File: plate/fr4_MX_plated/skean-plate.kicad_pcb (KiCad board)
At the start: 2 copper layers, 153.2 x 95.3 mm, 32 parts, among them K1 KEYSW, K10 KEYSW, K11 KEYSW, K12 KEYSW, K13 KEYSW, K14 KEYSW, K15 KEYSW, K16 KEYSW, K17 KEYSW, K18 KEYSW, K19 KEYSW, K2 KEYSW, K20 KEYSW, K21 KEYSW, K22 KEYSW, K3 KEYSW, K4 KEYSW, K5 KEYSW, K6 KEYSW, K7 KEYSW, K8 KEYSW, K9 KEYSW

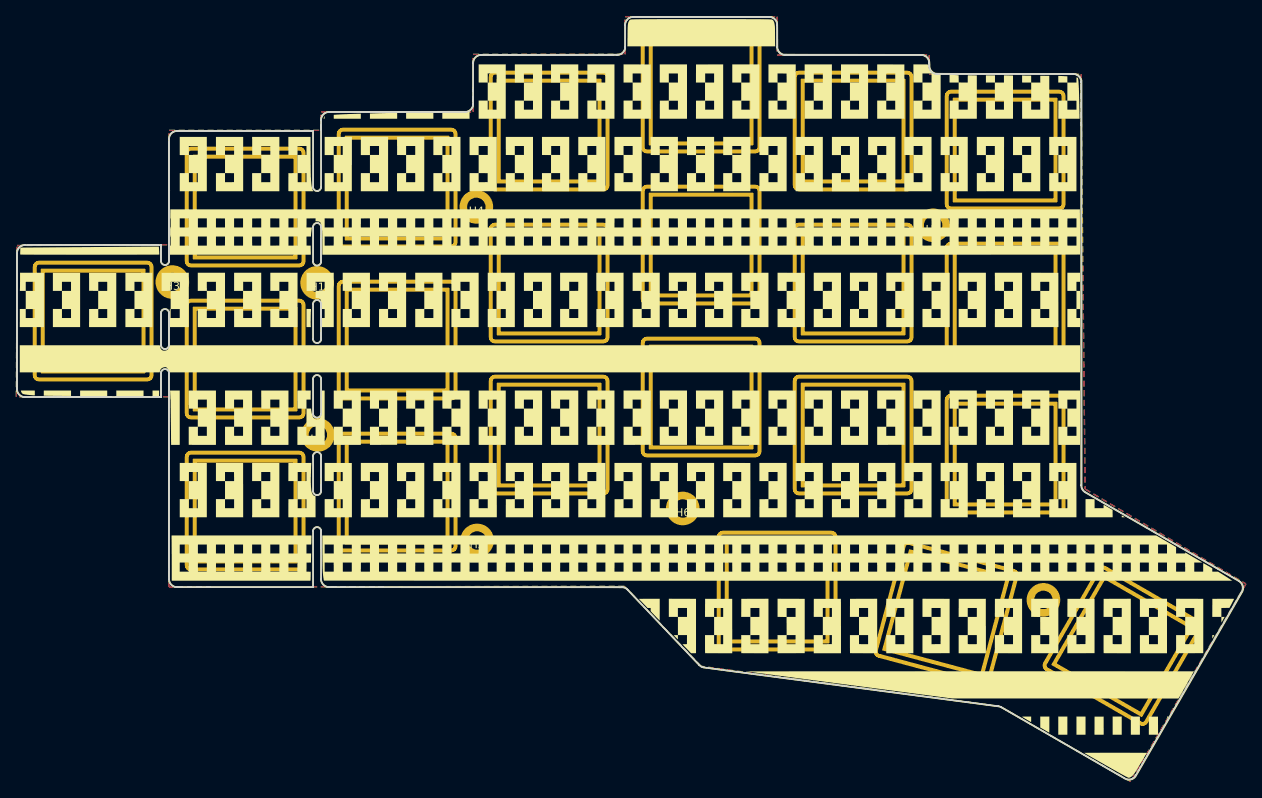
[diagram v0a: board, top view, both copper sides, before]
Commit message: V0.3 case files
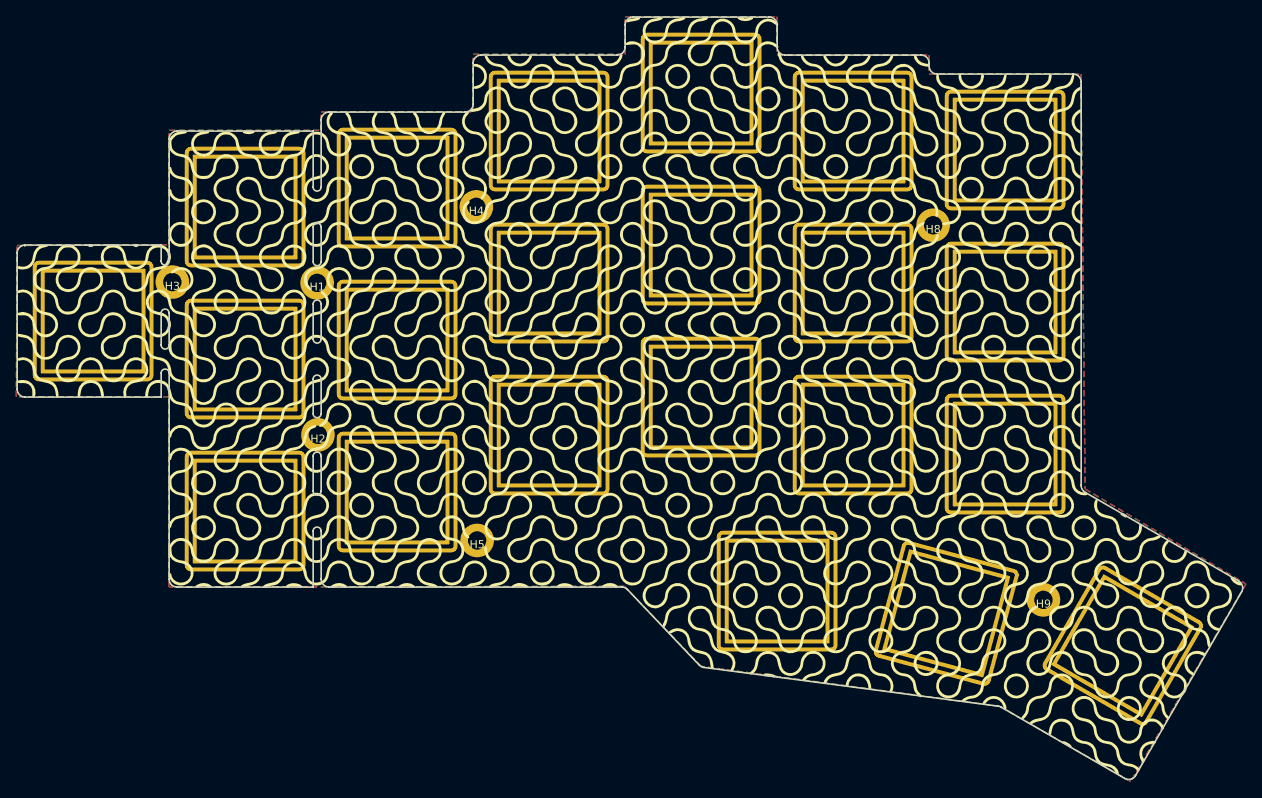
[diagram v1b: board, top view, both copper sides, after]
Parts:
- removed the G*** at (90.8, 62.0) (x2)
- removed H6: MountingHole, kbd:M2_Hole_TH
- added G***: LOGO, Silks:skean_truchet_back, F.Cu at (91.2, 61.6)
- added REF**: LOGO, Silks:skean_truchet, F.Cu at (90.8, 61.6)
